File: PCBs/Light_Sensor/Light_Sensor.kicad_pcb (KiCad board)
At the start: 2 copper layers, 5 parts, among them J2 Conn_01x03

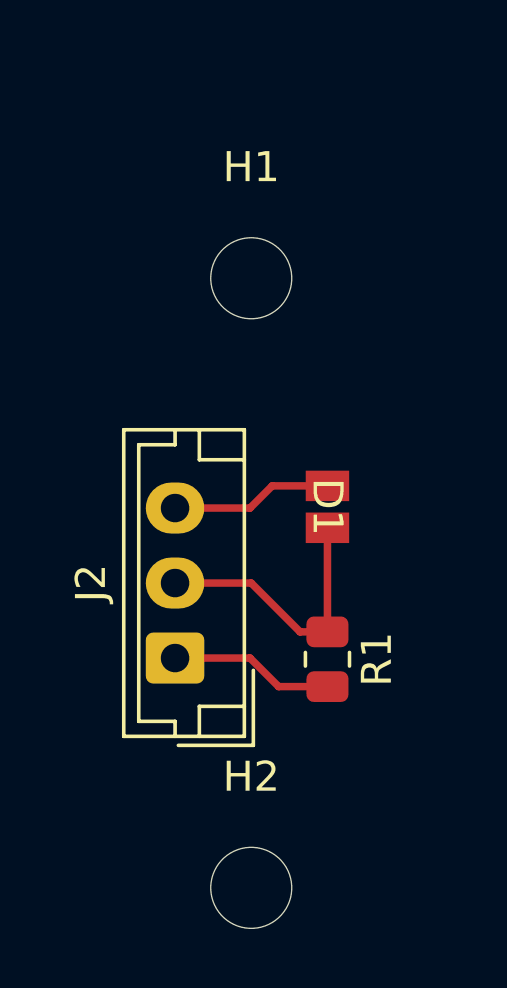
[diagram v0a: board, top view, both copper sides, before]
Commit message: latest PCBs
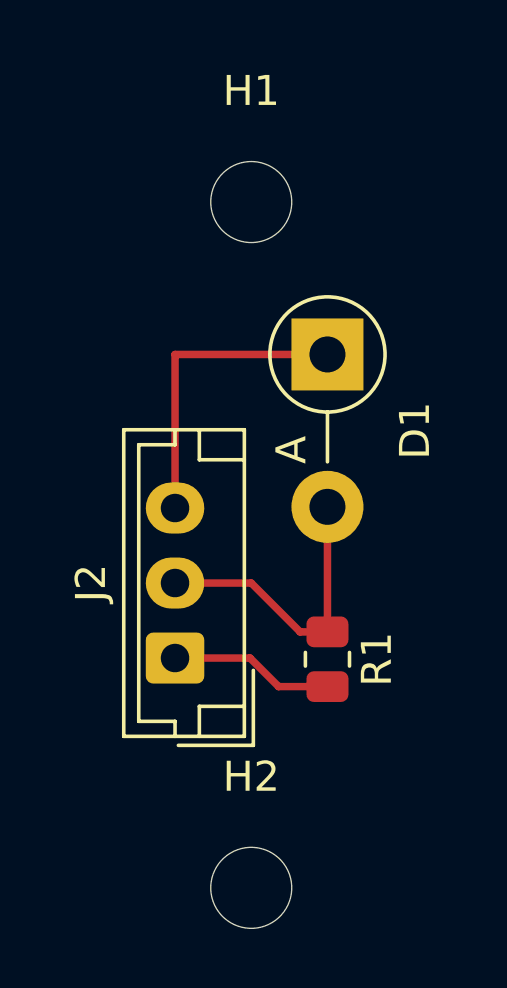
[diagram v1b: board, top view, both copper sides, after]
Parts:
- D1: footprint Artisyn_Components:DIODE_0805 -> Diode_THT:D_DO-15_P5.08mm_Vertical_AnodeUp
- moved D1 5.08 mm to (149.9, 78.7)
- moved H1 2.54 mm to (147.3, 73.7)
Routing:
- net VCC: track 5.39 -> 10.2 mm
- net Net-(D1-A): track 9.22 -> 9.92 mm
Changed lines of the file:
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@@
     (pad "" np_thru_hole circle (at 0 0) (size 2.7 2.7) (drill 2.7) (layers "*.Cu" "*.Mask"))
   )
-  (footprint "Artisyn_Components:DIODE_0805" (layer "F.Cu")
-    (at 149.86 83.82 -90)
-    (tags "TEMD7000X01 ")
+  (footprint "Diode_THT:D_DO-15_P5.08mm_Vertical_AnodeUp" (layer "F.Cu")
+    (at 149.86 78.74 -90)
+    (descr "Diode, DO-15 series, Axial, Vertical, pin pitch=5.08mm, , length*diameter=7.6*3.6mm^2, , http://www.diodes.com/_files/packages/DO-15.pdf")
+    (tags "Diode DO-15 series Axial Vertical pin pitch 5.08mm  length 7.6mm diameter 3.6mm")
     (property "Sheetfile" "Light_Sensor.kicad_sch")
     (property "Sheetname" "")
     (property "ki_description" "Photodiode")
     (property "ki_keywords" "photodiode diode opto")
-    (attr smd)
-    (fp_text reference "D1" (at 0 0 -90 unlocked) (layer "F.SilkS")
-        (effects (font (size 1 1) (thickness 0.15)))
-    )
-    (fp_text value "D_Photo" (at 0 -2.54 -90 unlocked) (layer "F.Fab")
-        (effects (font (size 1 1) (thickness 0.15)))
-    )
-    (fp_text user "${REFERENCE}" (at 0 0 -90 unlocked) (layer "F.Fab")
-        (effects (font (size 1 1) (thickness 0.15)))
-    )
-    (fp_line (start -1.4605 -0.9779) (end 1.4605 -0.9779)
-      (stroke (width 0.1524) (type solid)) (layer "F.CrtYd"))
-    (fp_line (start -1.4605 0.9779) (end -1.4605 -0.9779)
-      (stroke (width 0.1524) (type solid)) (layer "F.CrtYd"))
-    (fp_line (start 1.4605 -0.9779) (end 1.4605 0.9779)
-      (stroke (width 0.1524) (type solid)) (layer "F.CrtYd"))
-    (fp_line (start 1.4605 0.9779) (end -1.4605 0.9779)
-      (stroke (width 0.1524) (type solid)) (layer "F.CrtYd"))
-    (fp_line (start -1.0033 -0.7239) (end -1.0033 0.7239)
-      (stroke (width 0.0254) (type solid)) (layer "F.Fab"))
-    (fp_line (start -1.0033 -0.7239) (end -1.0033 0.7239)
-      (stroke (width 0.0254) (type solid)) (layer "F.Fab"))
-    (fp_line (start -1.0033 0.7239) (end -0.1905 0.7239)
-      (stroke (width 0.0254) (type solid)) (layer "F.Fab"))
-    (fp_line (start -1.0033 0.7239) (end 1.0033 0.7239)
-      (stroke (width 0.0254) (type solid)) (layer "F.Fab"))
-    (fp_line (start -0.1905 -0.7239) (end -1.0033 -0.7239)
-      (stroke (width 0.0254) (type solid)) (layer "F.Fab"))
-    (fp_line (start -0.1905 0.7239) (end -0.1905 -0.7239)
-      (stroke (width 0.0254) (type solid)) (layer "F.Fab"))
-    (fp_line (start 0.1905 -0.7239) (end 0.1905 0.7239)
-      (stroke (width 0.0254) (type solid)) (layer "F.Fab"))
-    (fp_line (start 0.1905 0.7239) (end 1.0033 0.7239)
-      (stroke (width 0.0254) (type solid)) (layer "F.Fab"))
-    (fp_line (start 1.0033 -0.7239) (end -1.0033 -0.7239)
-      (stroke (width 0.0254) (type solid)) (layer "F.Fab"))
-    (fp_line (start 1.0033 -0.7239) (end 0.1905 -0.7239)
-      (stroke (width 0.0254) (type solid)) (layer "F.Fab"))
-    (fp_line (start 1.0033 0.7239) (end 1.0033 -0.7239)
-      (stroke (width 0.0254) (type solid)) (layer "F.Fab"))
-    (fp_line (start 1.0033 0.7239) (end 1.0033 -0.7239)
-      (stroke (width 0.0254) (type solid)) (layer "F.Fab"))
-    (pad "1" smd rect (at -0.6985 0 270) (size 1.016 1.4478) (layers "F.Cu" "F.Paste" "F.Mask")
+    (attr through_hole)
+    (fp_text reference "D1" (at 2.54 -2.92 -90) (layer "F.SilkS")
+        (effects (font (size 1 1) (thickness 0.15)))
+    )
+    (fp_text value "D_Photo" (at 2.54 2.92 -90) (layer "F.Fab")
+        (effects (font (size 1 1) (thickness 0.15)))
+    )
+    (fp_text user "A" (at 3.18 1.2 -90) (layer "F.SilkS")
+        (effects (font (size 1 1) (thickness 0.15)))
+    )
+    (fp_text user "A" (at 3.18 1.2 -90) (layer "F.Fab")
+        (effects (font (size 1 1) (thickness 0.15)))
+    )
+    (fp_text user "${REFERENCE}" (at 2.54 -2.92 -90) (layer "F.Fab")
+        (effects (font (size 1 1) (thickness 0.15)))
+    )
+    (fp_line (start 1.92 0) (end 3.58 0)
+      (stroke (width 0.12) (type solid)) (layer "F.SilkS"))
+    (fp_circle (center 0 0) (end 1.92 0)
+      (stroke (width 0.12) (type solid)) (fill none) (layer "F.SilkS"))
+    (fp_line (start -2.05 -2.05) (end -2.05 2.05)
+      (stroke (width 0.05) (type solid)) (layer "F.CrtYd"))
+    (fp_line (start -2.05 2.05) (end 6.53 2.05)
+      (stroke (width 0.05) (type solid)) (layer "F.CrtYd"))
+    (fp_line (start 6.53 -2.05) (end -2.05 -2.05)
+      (stroke (width 0.05) (type solid)) (layer "F.CrtYd"))
+    (fp_line (start 6.53 2.05) (end 6.53 -2.05)
+      (stroke (width 0.05) (type solid)) (layer "F.CrtYd"))
+    (fp_line (start 0 0) (end 5.08 0)
+      (stroke (width 0.1) (type solid)) (layer "F.Fab"))
+    (fp_circle (center 0 0) (end 1.8 0)
+      (stroke (width 0.1) (type solid)) (fill none) (layer "F.Fab"))
+    (pad "1" thru_hole rect (at 0 0 270) (size 2.4 2.4) (drill 1.2) (layers "*.Cu" "*.Mask")
       (net 1 "VCC") (pinfunction "K") (pintype "passive"))
-    (pad "2" smd rect (at 0.6985 0 270) (size 1.016 1.4478) (layers "F.Cu" "F.Paste" "F.Mask")
+    (pad "2" thru_hole oval (at 5.08 0 270) (size 2.4 2.4) (drill 1.2) (layers "*.Cu" "*.Mask")
       (net 2 "Net-(D1-A)") (pinfunction "A") (pintype "passive"))
-    (zone (net 0) (net_name "") (layer "F.Cu") (hatch full 0.508)
-      (connect_pads (clearance 0))
-      (min_thickness 0.254) (filled_areas_thickness no)
-      (keepout (tracks not_allowed) (vias not_allowed) (pads allowed) (copperpour not_allowed) (footprints allowed))
-      (fill (thermal_gap 0.508) (thermal_bridge_width 0.508))
-      (polygon
-        (pts
-          (xy 150.5331 83.6803)
-          (xy 150.5331 83.9597)
-          (xy 149.1869 83.9597)
-          (xy 149.1869 83.6803)
-        )
-      )
+    (model "${KICAD6_3DMODEL_DIR}/Diode_THT.3dshapes/D_DO-15_P5.08mm_Vertical_AnodeUp.wrl"
+      (offset (xyz 0 0 0))
+      (scale (xyz 1 1 1))
+      (rotate (xyz 0 0 0))
     )
   )
   (footprint "MountingHole:MountingHole_2.7mm" (layer "F.Cu")
-    (at 147.32 76.2)
+    (at 147.32 73.66)
     (descr "Mounting Hole 2.7mm, no annular")
     (tags "mounting hole 2.7mm no annular")
@@
     )
   )
-  (segment (start 149.86 83.1215) (end 148.0185 83.1215) (width 0.25) (layer "F.Cu") (net 1))
-  (segment (start 148.0185 83.1215) (end 147.28 83.86) (width 0.25) (layer "F.Cu") (net 1))
-  (segment (start 147.28 83.86) (end 144.78 83.86) (width 0.25) (layer "F.Cu") (net 1))
+  (segment (start 144.78 83.86) (end 144.78 78.74) (width 0.25) (layer "F.Cu") (net 1))
+  (segment (start 144.78 78.74) (end 149.86 78.74) (width 0.25) (layer "F.Cu") (net 1))
+  (segment (start 149.86 83.82) (end 149.86 87.9875) (width 0.25) (layer "F.Cu") (net 2))
   (segment (start 149.86 87.9875) (end 148.9475 87.9875) (width 0.25) (layer "F.Cu") (net 2))
   (segment (start 147.32 86.36) (end 144.78 86.36) (width 0.25) (layer "F.Cu") (net 2))
-  (segment (start 149.86 87.9875) (end 149.86 84.5185) (width 0.25) (layer "F.Cu") (net 2))
   (segment (start 148.9475 87.9875) (end 147.32 86.36) (width 0.25) (layer "F.Cu") (net 2))
   (segment (start 147.28 88.86) (end 144.78 88.86) (width 0.25) (layer "F.Cu") (net 3))
